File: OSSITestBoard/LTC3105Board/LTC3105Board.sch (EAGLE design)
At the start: 20 parts, among them U1 LT3105-MS

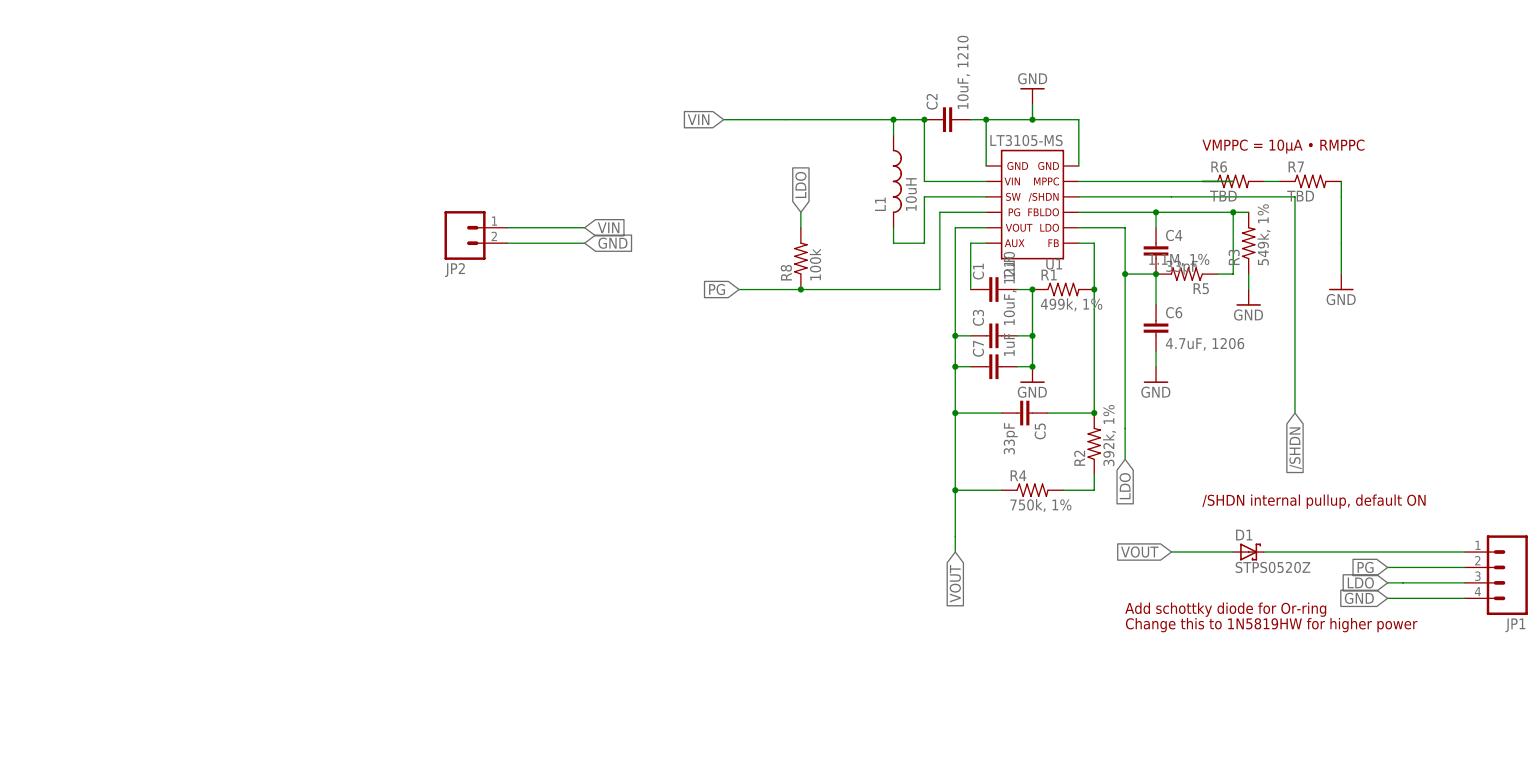
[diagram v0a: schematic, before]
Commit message: LTC3105 board notes added
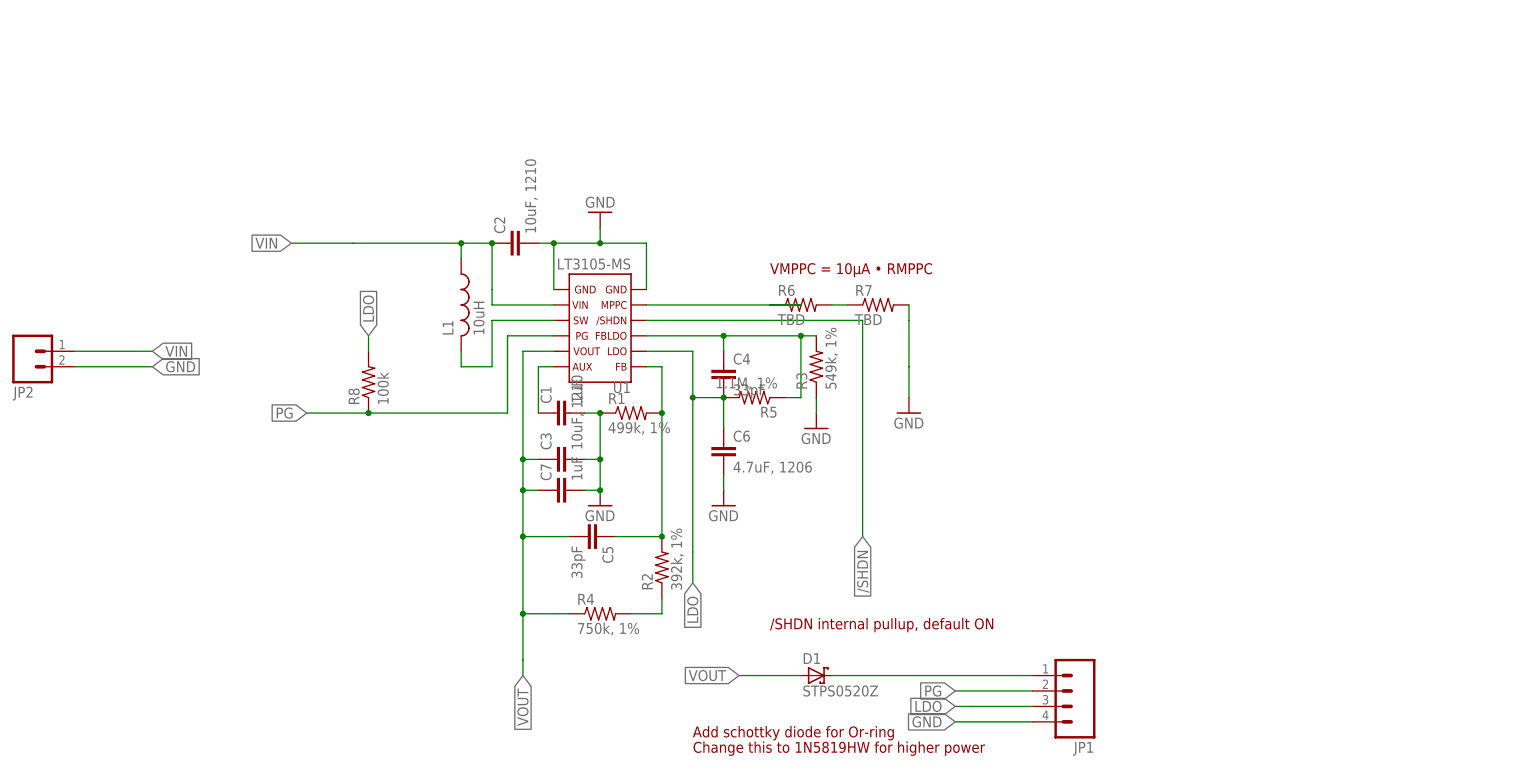
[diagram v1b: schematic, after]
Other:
- moved on the sheet: C1, C2, C3, C4, C5, C6, C7, D1, JP1, JP2, L1, R1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
